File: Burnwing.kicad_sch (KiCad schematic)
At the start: 41 parts, among them J1 USB Type C, J2 Conn_01x06_MountingPin, J3 Conn_01x02_Pin, Q1 NCV8402ADDR2G, Q2 AONR21307, U1 HUSB238

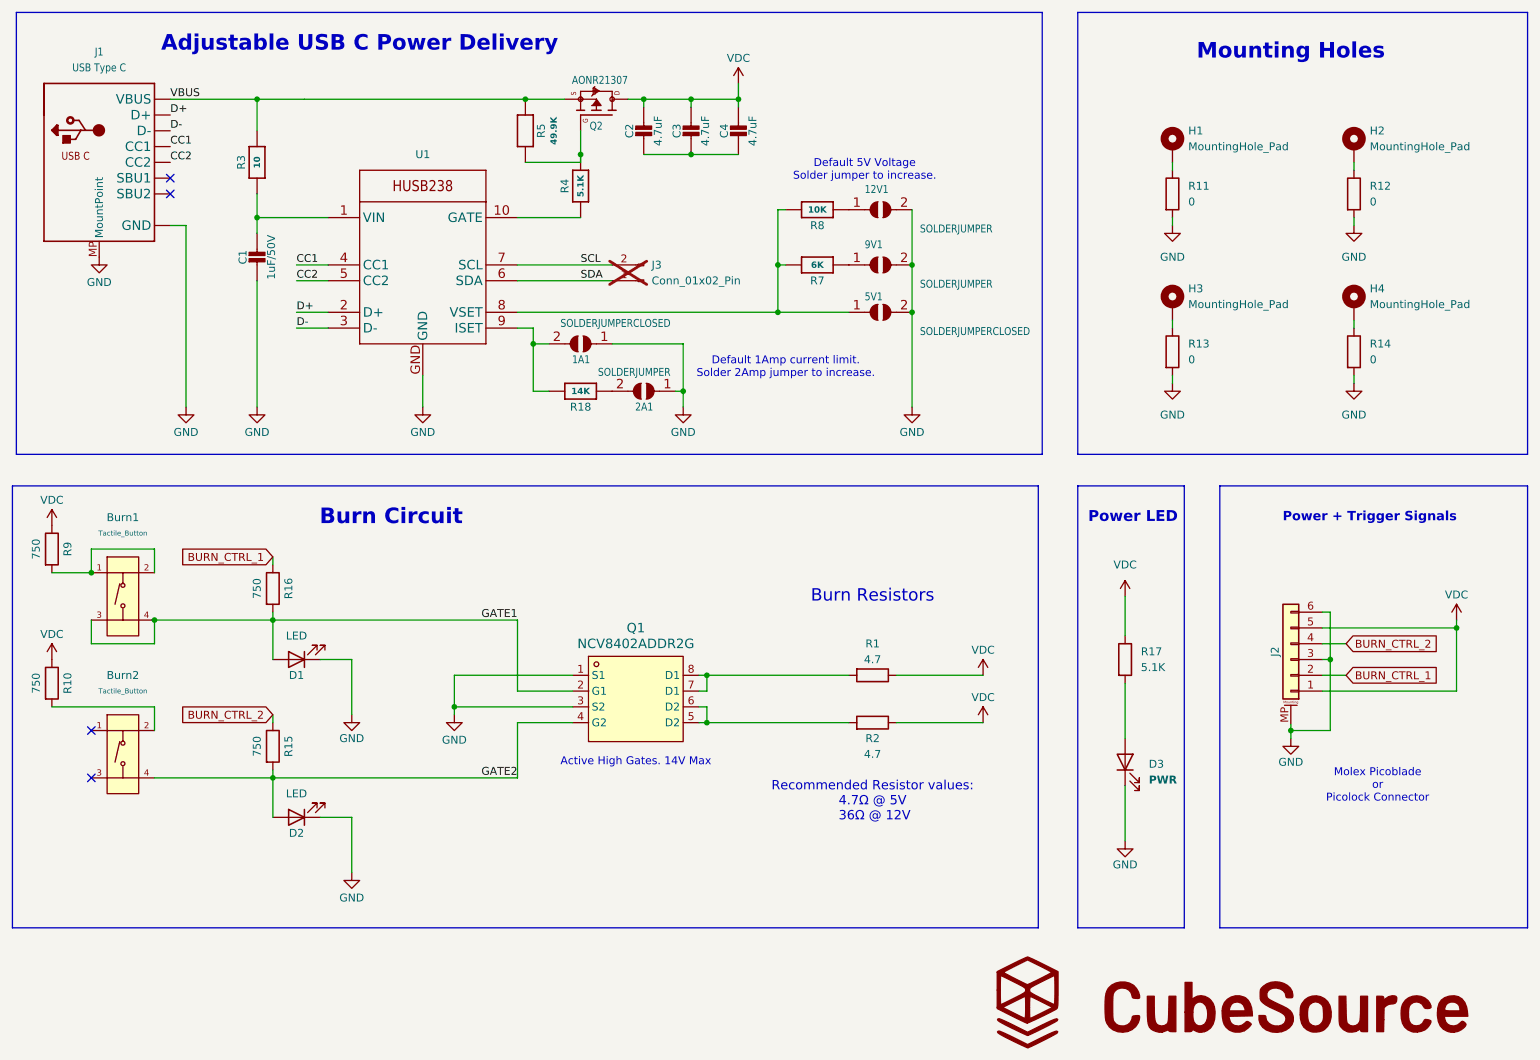
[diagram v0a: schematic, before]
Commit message: 4 layer v3 template
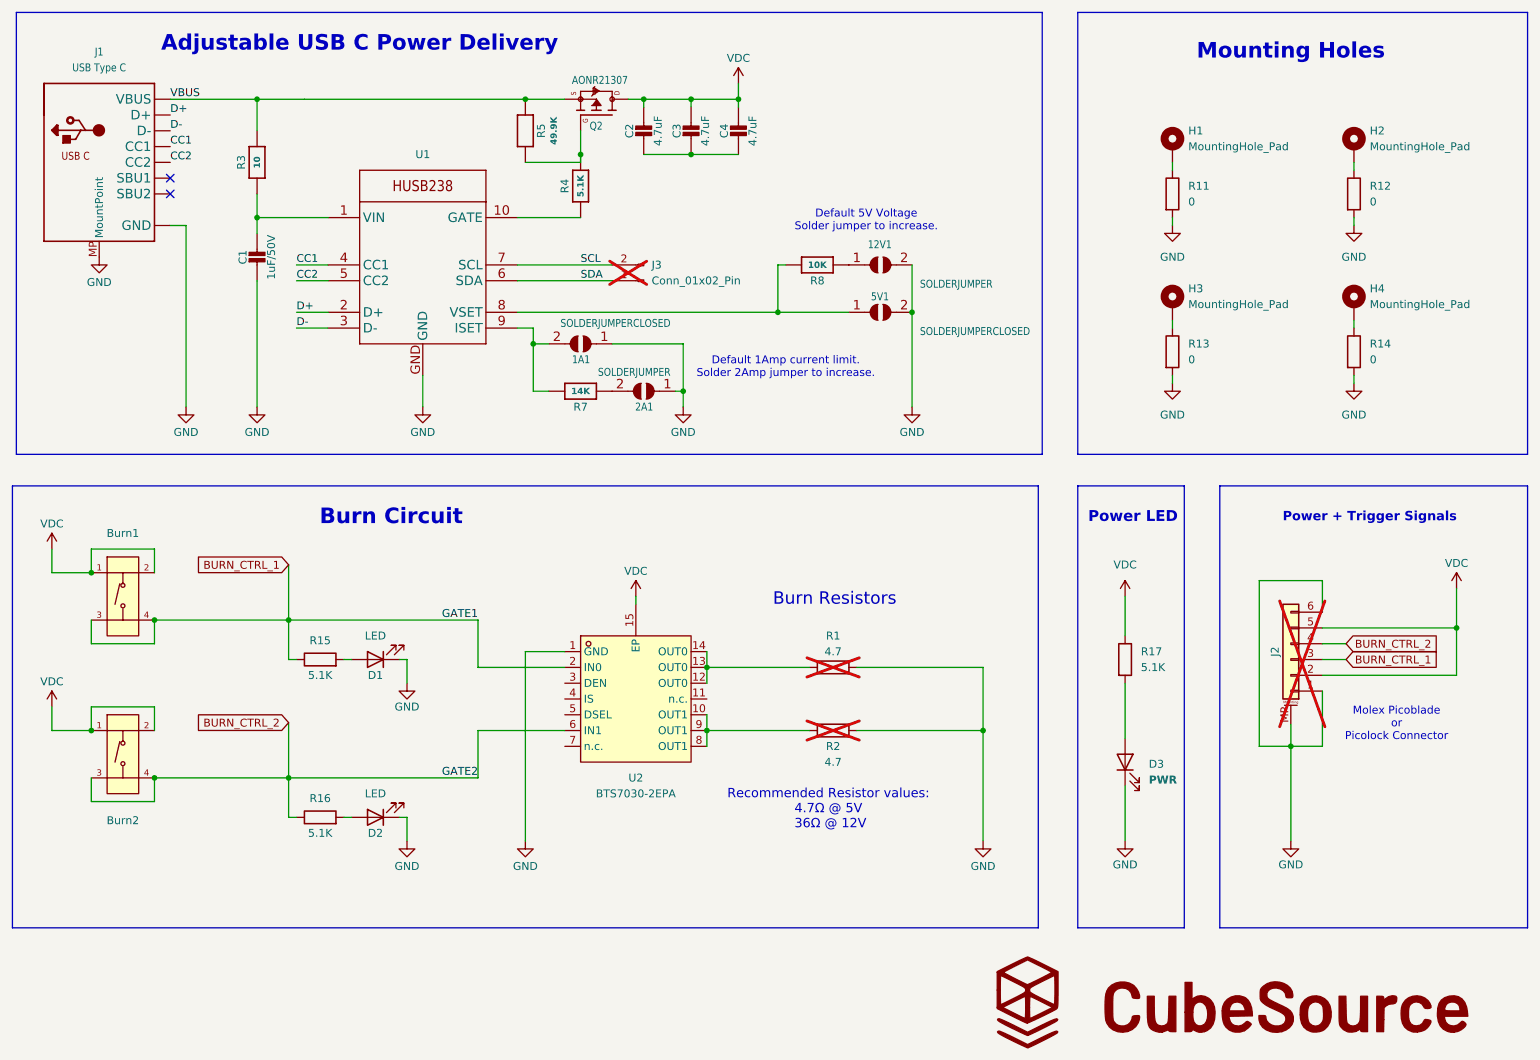
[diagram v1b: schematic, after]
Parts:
- removed 9V1: SOLDERJUMPER, Library:SOLDERJUMPER_ARROW_NOPASTE, symbol Library:microbuilder_SOLDERJUMPER
- removed Q1: NCV8402ADDR2G, EasyEDA:SOIC-8_L4.9-W3.9-P1.27-LS6.0-BL, symbol EasyEDA:NCV8402ADDR2G
- removed R10, R9: 750, Resistor_SMD:R_0603_1608Metric_Pad0.98x0.95mm_HandSolder, symbol Library:R
- removed R7: 6K, Resistor_SMD:R_0603_1608Metric_Pad0.98x0.95mm_HandSolder, symbol Library:microbuilder_RESISTOR_0603_NOOUT
- added U2: BTS7030-2EPA, EasyEDA:PG-TSDSO-14_L4.9-W3.9-P0.65-LS6.0-BL-EP, symbol EasyEDA:BTS7030-2EPA
- Burn1, Burn2: value Tactile_Button -> KEY-SMD_4P-L6.0-W6.0-P4.50-LS9.5-BR; footprint PCM_JLCPCB:SW-SMD_4P-L5.1-W5.1-P3.70-LS6.5-TL-2 -> EasyEDA:KEY-SMD_4P-L6.0-W6.0-P4.50-LS9.5-BR; Actuator Style Round Button -> (none); Actuator/Cap Color Golden -> (none); Attrition Qty 5 -> (none); Category Switches,Tactile Switches -> (none); Circuit SPST -> (none); Class Basic Component -> (none); Contact Current 50mA -> (none); LCSC C318884 -> (none); Manufacturer XKB Connectivity -> (none); Mechanical Life 100000 Times -> (none); Minimum Qty 10 -> (none); Mounting Style Brick nogging -> (none); Operating Force 160gf -> (none); Operating Temperature -30°C~+85°C -> (none); Part TS-1187A-B-A-B -> (none); Price 0.025USD -> (none); Process SMT -> (none); Stock 433660 -> (none); Strike Gundam NO -> (none); Switch Height 1.5mm -> (none); Switch Length 5.1mm -> (none); Switch Width 5.1mm -> (none); Voltage Rating (Dc) 12V -> (none); With Lamp No -> (none)
- C1: footprint Capacitor_SMD:C_0805_2012Metric_Pad1.18x1.45mm_HandSolder -> Library:C_0805_2012Metric_Pad1.18x1.45mm_HandSolder; LCSC (none) -> C28323
- C2, C3, C4: footprint Capacitor_SMD:C_0805_2012Metric_Pad1.18x1.45mm_HandSolder -> Library:C_0805_2012Metric_Pad1.18x1.45mm_HandSolder; LCSC (none) -> C437557
- D1, D2, D3: footprint LED_SMD:LED_0603_1608Metric_Pad1.05x0.95mm_HandSolder -> Library:LED_0603_1608Metric_Pad1.05x0.95mm_HandSolder; LCSC (none) -> C94868
- H1, H2, H3, H4: footprint MountingHole:MountingHole_2.2mm_M2_Pad -> Library:MountingHole_2.2mm_M2_Pad
- J1: LCSC (none) -> C2988369
- J2: footprint Connector_Molex:Molex_PicoBlade_53261-0671_1x06-1MP_P1.25mm_Horizontal -> Library:Molex_PicoBlade_53261-0671_1x06-1MP_P1.25mm_Horizontal; Labels (none) -> +; now not fitted; now left out of the parts list
- J3: footprint Connector_PinHeader_1.00mm:PinHeader_1x02_P1.00mm_Vertical -> Library:PinHeader_1x02_P1.00mm_Vertical
- Q2: LCSC (none) -> C3277813
- R1, R2: now not fitted; now left out of the parts list
- R11: footprint Resistor_SMD:R_0603_1608Metric_Pad0.98x0.95mm_HandSolder -> Library:R_0603_1608Metric_Pad0.98x0.95mm_HandSolder; LCSC (none) -> C100044
- R12, R13, R14: footprint Resistor_SMD:R_0603_1608Metric_Pad0.98x0.95mm_HandSolder -> Library:R_0603_1608Metric_Pad0.98x0.95mm_HandSolder
- R15, R16: value 750 -> 5.1K; footprint Resistor_SMD:R_0603_1608Metric_Pad0.98x0.95mm_HandSolder -> Library:R_0603_1608Metric_Pad0.98x0.95mm_HandSolder; LCSC (none) -> C105580
- R17, R4: footprint Resistor_SMD:R_0603_1608Metric_Pad0.98x0.95mm_HandSolder -> Library:R_0603_1608Metric_Pad0.98x0.95mm_HandSolder; LCSC (none) -> C105580
- R3: footprint Resistor_SMD:R_0603_1608Metric_Pad0.98x0.95mm_HandSolder -> Library:R_0603_1608Metric_Pad0.98x0.95mm_HandSolder; LCSC (none) -> C203240
- R5: footprint Resistor_SMD:R_0603_1608Metric_Pad0.98x0.95mm_HandSolder -> Library:R_0603_1608Metric_Pad0.98x0.95mm_HandSolder; LCSC (none) -> C705780
- R7: renamed from R18; footprint Resistor_SMD:R_0603_1608Metric_Pad0.98x0.95mm_HandSolder -> Library:R_0603_1608Metric_Pad0.98x0.95mm_HandSolder; LCSC (none) -> C105580
- R8: footprint Resistor_SMD:R_0603_1608Metric_Pad0.98x0.95mm_HandSolder -> Library:R_0603_1608Metric_Pad0.98x0.95mm_HandSolder; LCSC (none) -> C95204
- U1: LCSC (none) -> C7471904
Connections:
- net BURN_CTRL_1: now also Burn1.3 (C), Burn1.4 (D), J2.3 (Pin_3), R15.1, U2.2 (IN0); no longer J2.2 (Pin_2), R16.1
- net BURN_CTRL_2: now also Burn2.3 (C), Burn2.4 (D), R16.1, U2.6 (IN1); no longer R15.1
- net GND: now also J2.1 (Pin_1), R1.1, R2.1, U2.1 (GND); no longer J2.3 (Pin_3)
- net VDC: now also Burn1.1 (A), Burn1.2 (B), Burn2.1 (A), Burn2.2 (B), J2.2 (Pin_2), U2.15 (EP); no longer J2.1 (Pin_1), R1.1, R2.1
- net at R2.2: now also U2.10 (OUT1), U2.8 (OUT1), U2.9 (OUT1)
- net at R1.2: now also U2.12 (OUT0), U2.13 (OUT0), U2.14 (OUT0)
- removed net GATE1: Burn1.3 (C), Burn1.4 (D), D1.2 (A), R16.2
- removed net GATE2: Burn2.4 (D), D2.2 (A), R15.2
- new net: D1.2 (A), R15.2
- new net: D2.2 (A), R16.2
- no-connect marks 4 -> 2
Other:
- note removed: "Active High Gates. 14V Max"
- moved on the sheet: 12V1, D1, D2, R8
